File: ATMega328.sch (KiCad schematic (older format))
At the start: 8 parts, among them J2 AVR-ISP-6, U1 ATmega328P-AU, Y1 Crystal_GND24

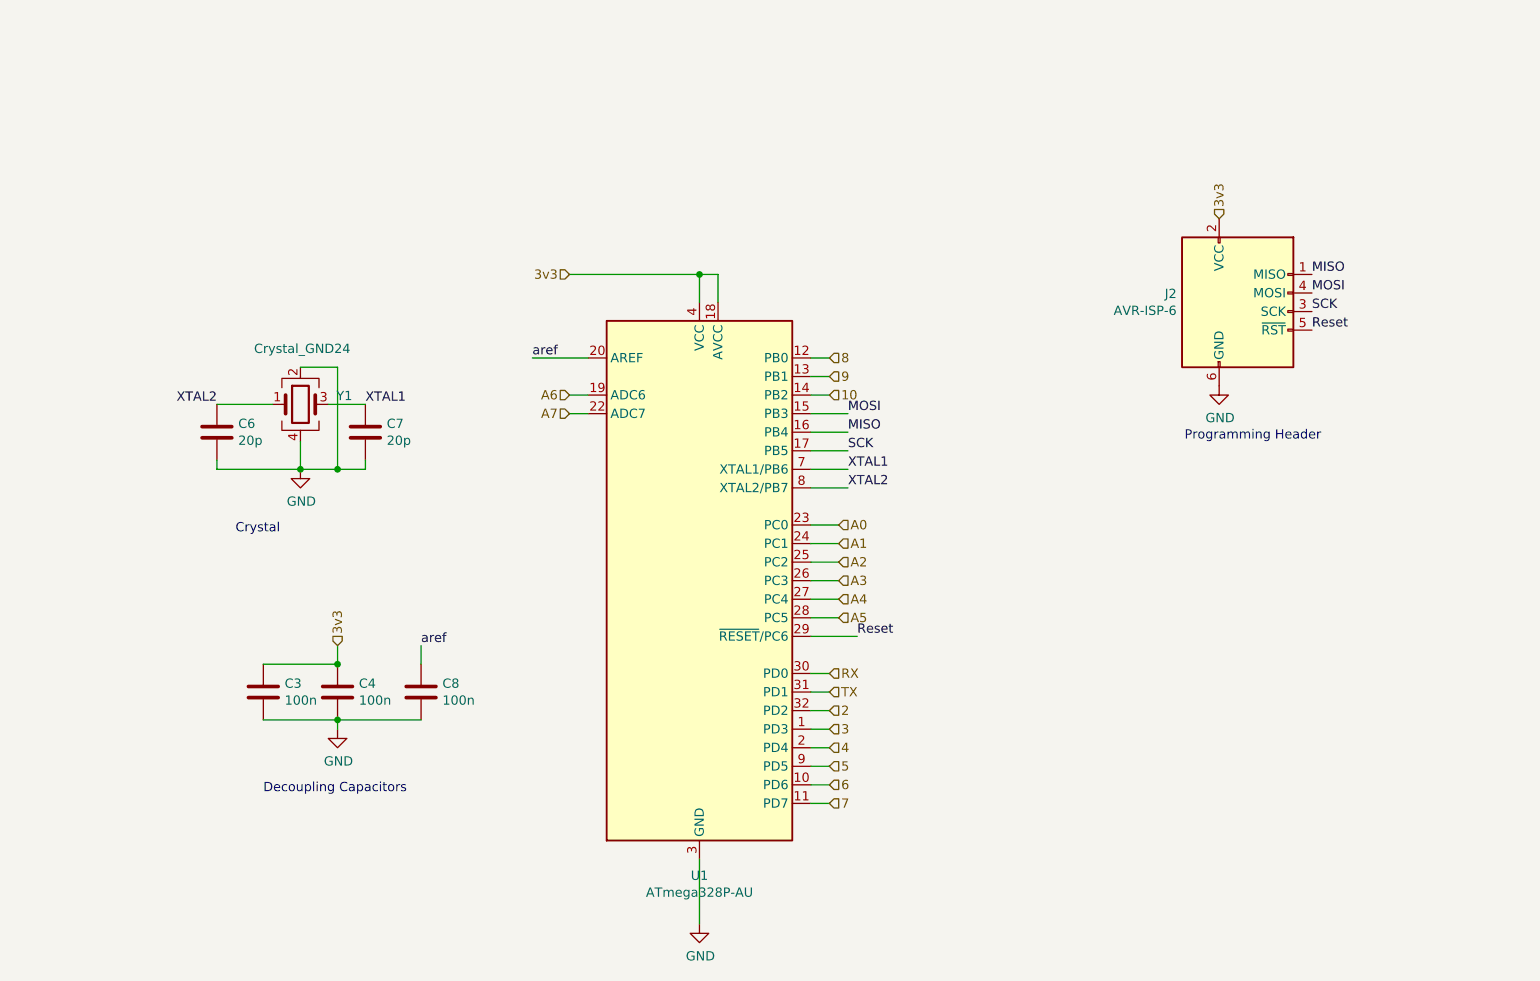
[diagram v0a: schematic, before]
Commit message: Version 0.3 prototype - Manufactured
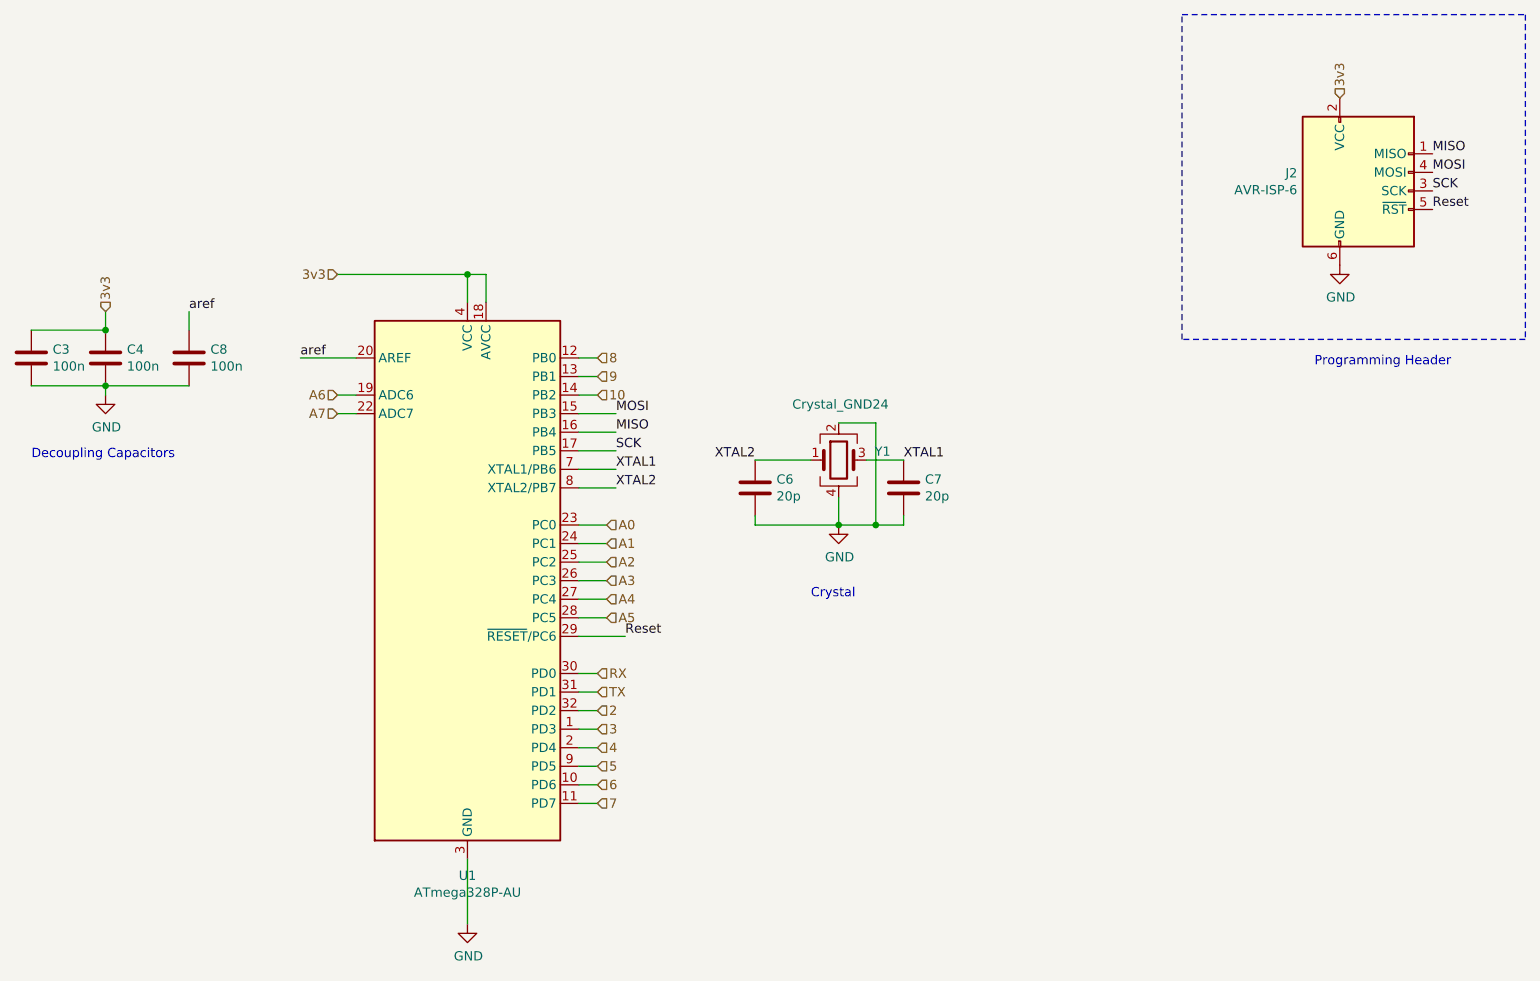
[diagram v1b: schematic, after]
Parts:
- C3, C4, C6, C7, C8: footprint Capacitor_SMD:C_0201_0603Metric -> Capacitor_SMD:C_0603_1608Metric
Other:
- moved on the sheet: C3, C4, C6, C7, C8, J2, U1, Y1
